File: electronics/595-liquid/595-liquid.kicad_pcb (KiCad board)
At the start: 2 copper layers, 6 parts, among them J1 Conn_01x05_Male, U1 74HC595, U2 RC1602A

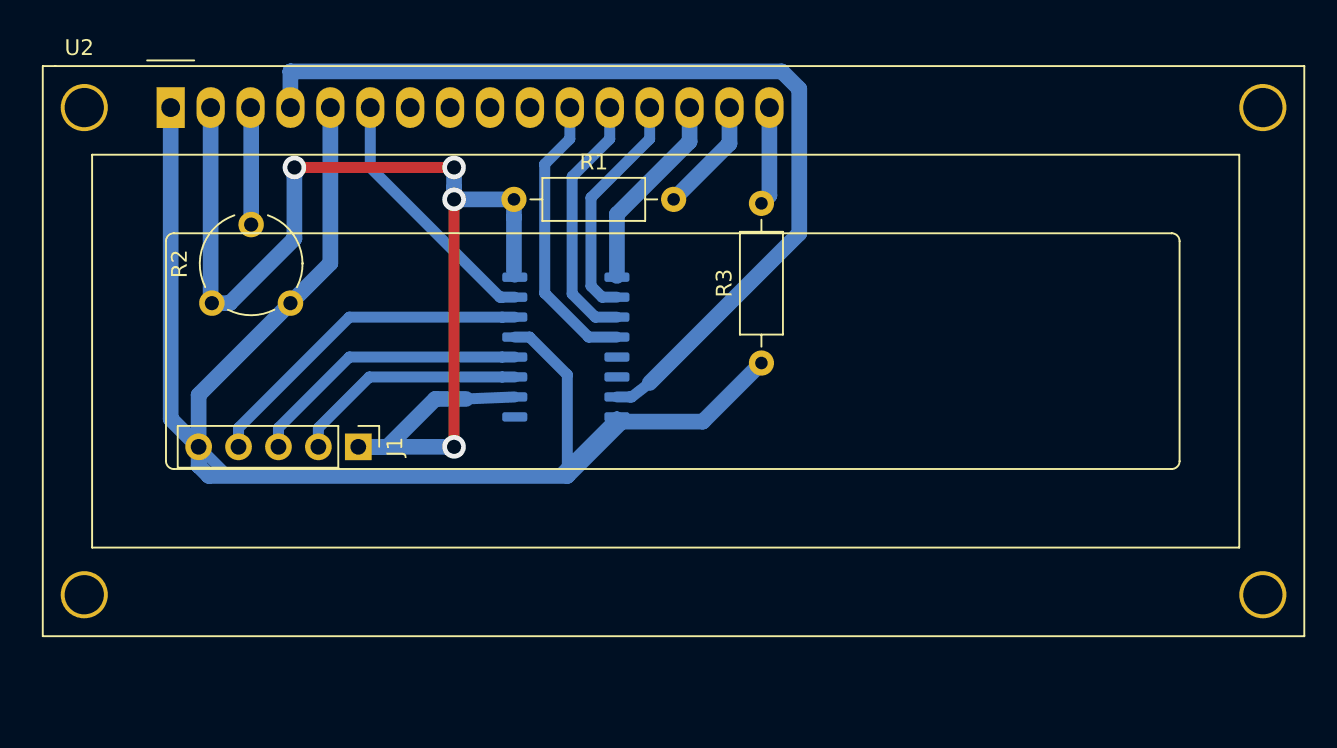
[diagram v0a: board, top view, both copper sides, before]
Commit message: Some changes
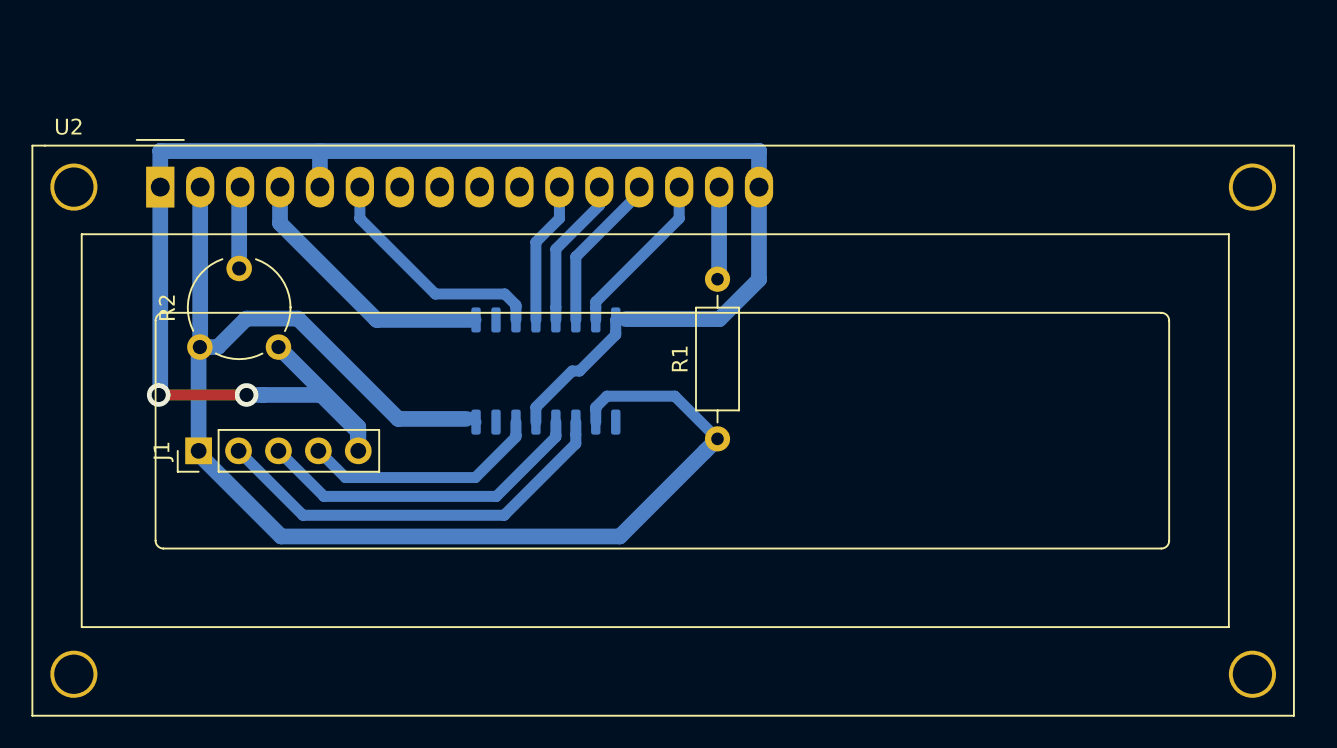
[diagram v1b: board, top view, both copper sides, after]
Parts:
- removed R3: 220, Resistor_THT:R_Axial_DIN0207_L6.3mm_D2.5mm_P10.16mm_Horizontal
- moved R1 20.0 mm to (130.6, 83.1), turned to 90 degrees
- moved J1 10.2 mm to (97.5, 83.8), turned to 90 degrees
- moved U2 5.10 mm to (95.1, 67.0)
- moved R2 2.90 mm to (102.6, 77.2)
- moved U1 1.98 mm to (119.6, 78.7), turned to 270 degrees
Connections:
- U1 pad 15: Net-(U1-Pad15) -> (no net)
- U1 pad 2: Net-(U1-Pad2) -> (no net)
- U1 pad 5: (no net) -> Net-(U1-Pad5)
- U1 pad 6: (no net) -> Net-(U1-Pad6)
- U2 pad 12: Net-(U1-Pad3) -> Net-(U1-Pad5)
- U2 pad 13: Net-(U1-Pad2) -> Net-(U1-Pad6)
- U2 pad 14: Net-(U1-Pad1) -> Net-(U1-Pad7)
- U2 pad 16: Net-(R3-Pad2) -> GND
- U2 pad 4: Net-(U1-Pad7) -> Net-(U1-Pad1)
- U2 pad 6: Net-(U1-Pad15) -> Net-(U1-Pad3)
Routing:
- net Net-(U1-Pad7): track 60.2 -> 10.7 mm
- net Net-(U1-Pad15): track 16.4 -> 0.00 mm
- net Net-(U1-Pad2): track 14.8 -> 0.00 mm
- net +5V: track 78.0 -> 90.3 mm, vias 4 -> 0
- net Net-(J1-Pad2): track 15.0 -> 26.4 mm
- net Net-(U1-Pad6): track 0.00 -> 10.1 mm
- net Net-(U1-Pad5): track 0.00 -> 9.60 mm
- net Net-(U1-Pad4): track 18.2 -> 9.07 mm
- net Net-(U1-Pad1): track 25.3 -> 17.3 mm
- net Net-(J1-Pad4): track 21.7 -> 15.3 mm
- net Net-(R3-Pad2): track 6.31 -> 0.00 mm
- net Net-(J1-Pad3): track 18.1 -> 21.4 mm
- net Net-(R2-Pad2): track 7.46 -> 5.20 mm
- net Net-(R1-Pad2): track 7.31 -> 5.90 mm
- net GND: track 150.0 -> 151.1 mm, vias 0 -> 2
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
